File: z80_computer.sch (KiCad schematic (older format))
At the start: 45 parts, among them J1 7-25v, SW1 RESET, U1 74HCT04, U2 NE555P, U3 LM2576HVS-ADJ, U4 74LS74, Y1 7.3728 MHz

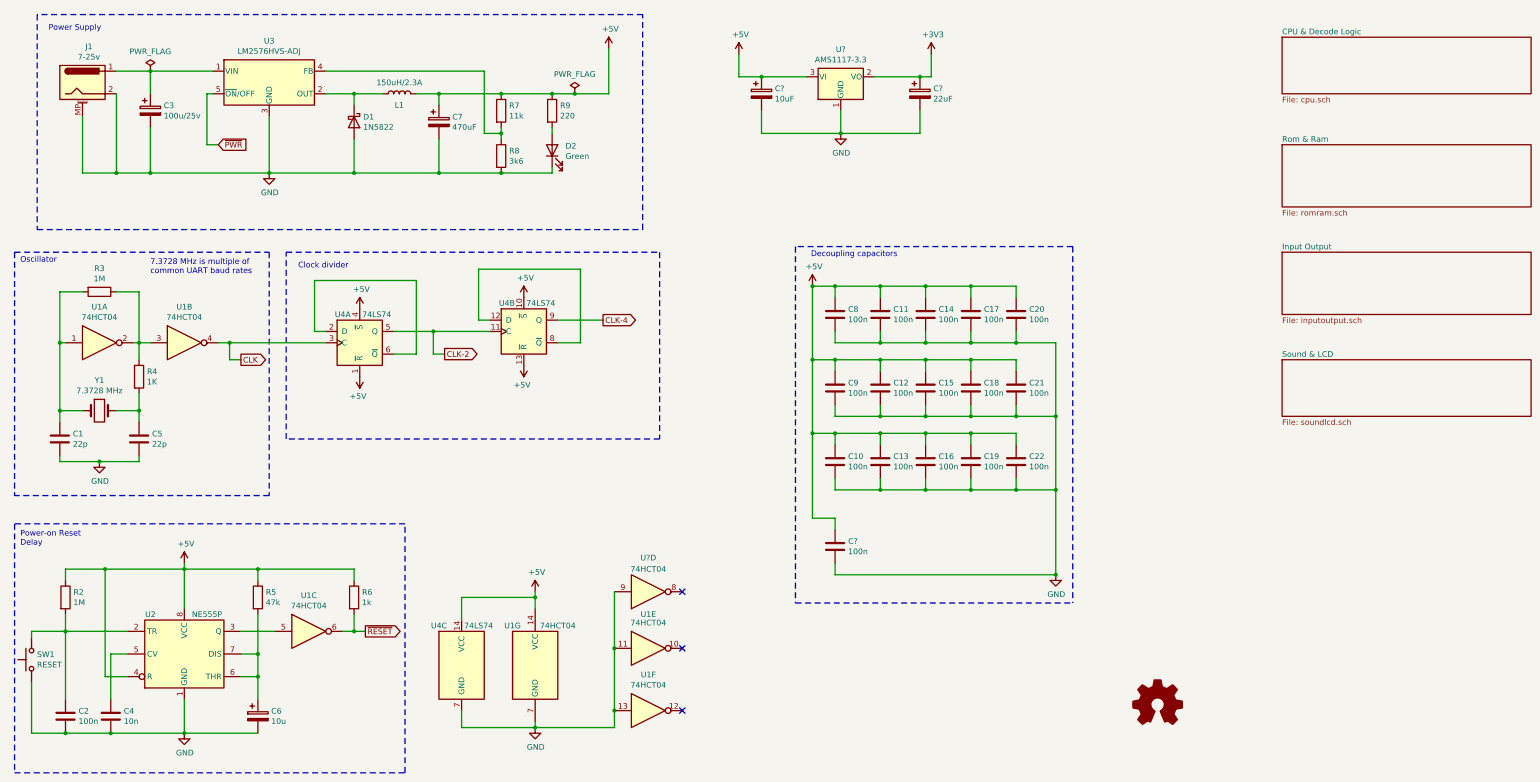
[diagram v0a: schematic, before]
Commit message: Updated schematic
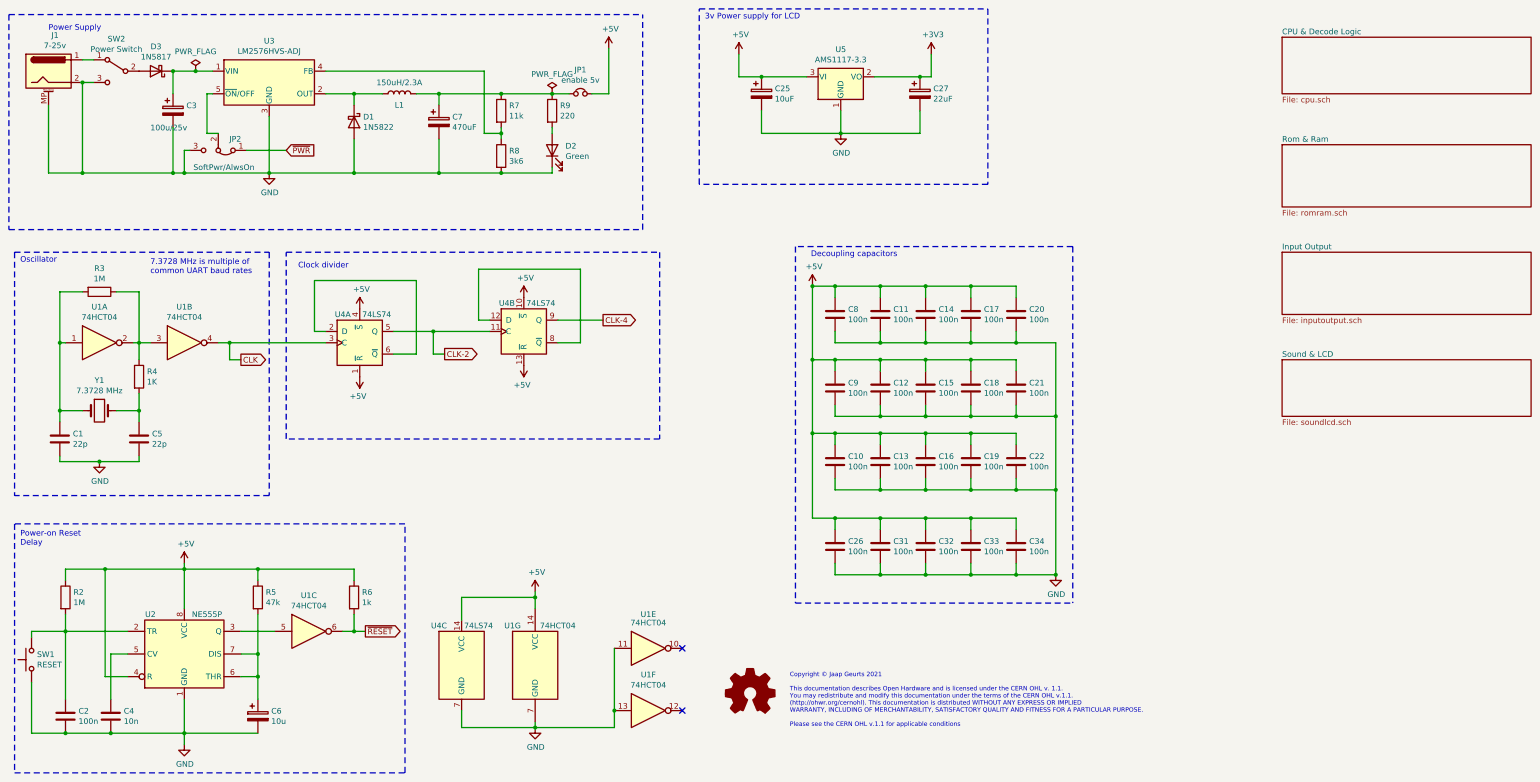
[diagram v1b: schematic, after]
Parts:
- removed U?: 74HCT04, Package_DIP:DIP-14_W7.62mm_Socket, symbol 74xx:74HCT04
- added C31, C32, C33, C34: 100n, symbol Device:C
- added D3: 1N5817, Diode_THT:D_DO-41_SOD81_P10.16mm_Horizontal, symbol Diode:1N5817
- added JP1: enable 5v, Connector_PinHeader_2.54mm:PinHeader_1x02_P2.54mm_Vertical, symbol Device:Jumper_NC_Small
- added JP2: SoftPwr/AlwsOn, Connector_PinHeader_2.54mm:PinHeader_1x03_P2.54mm_Vertical, symbol Jumper:Jumper_3_Bridged12
- added SW2: Power Switch, Button_Switch_THT:SW_Slide_1P2T_CK_OS102011MS2Q, symbol Switch:SW_SPDT
- D2: footprint (none) -> LED_THT:LED_D5.0mm
- L1: footprint (none) -> Inductor_THT:L_Radial_D10.0mm_P5.00mm_Fastron_07M
- R2, R3, R4, R5, R6, R7, R8, R9: footprint (none) -> Resistor_THT:R_Axial_DIN0207_L6.3mm_D2.5mm_P10.16mm_Horizontal
- U4: footprint (none) -> Package_DIP:DIP-14_W7.62mm_Socket_LongPads
- Y1: footprint (none) -> Crystal:Crystal_HC49-U_Vertical
- gave numbers to parts that had none: 4
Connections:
- net +5V: now also C31.1, C32.1, C33.1, C34.1, JP1.2; no longer C7.1, L1.2, R7.1, R9.1
- net GND: now also C31.2, C32.2, C33.2, C34.2, JP2.3 (B), SW2.3 (C)
- net ~PWR: now also JP2.1 (A); no longer U3.5 (~ON~/OFF)
- net at C3.1, U3.1 (VIN): now also D3.1 (K); no longer J1.1
- new net: JP2.2 (C), U3.5 (~ON~/OFF)
- new net: J1.1, SW2.1 (A)
- new net: C7.1, JP1.1, L1.2, R7.1, R9.1
- new net: D3.2 (A), SW2.2 (B)
- no-connect marks 3 -> 2
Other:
- note added: "3v Power supply for LCD"
- note added: "Copyright © Jaap Geurts 2021\n\nThis documentation describes Open Hardware and is licensed under the CERN OHL v. 1.1.\nYou may redistribute and modify this documentation under the terms of the CERN OHL v.1.1.\n(http://ohwr.org/cernohl). This documentation is distributed WITHOUT ANY EXPRESS OR IMPLIED\nWARRANTY, INCLUDING OF MERCHANTABILITY, SATISFACTORY QUALITY AND FITNESS FOR A PARTICULAR PURPOS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"
- moved on the sheet: C3, J1
